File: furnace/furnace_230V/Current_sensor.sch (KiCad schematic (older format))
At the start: 14 parts, among them T1 ZMCT103C

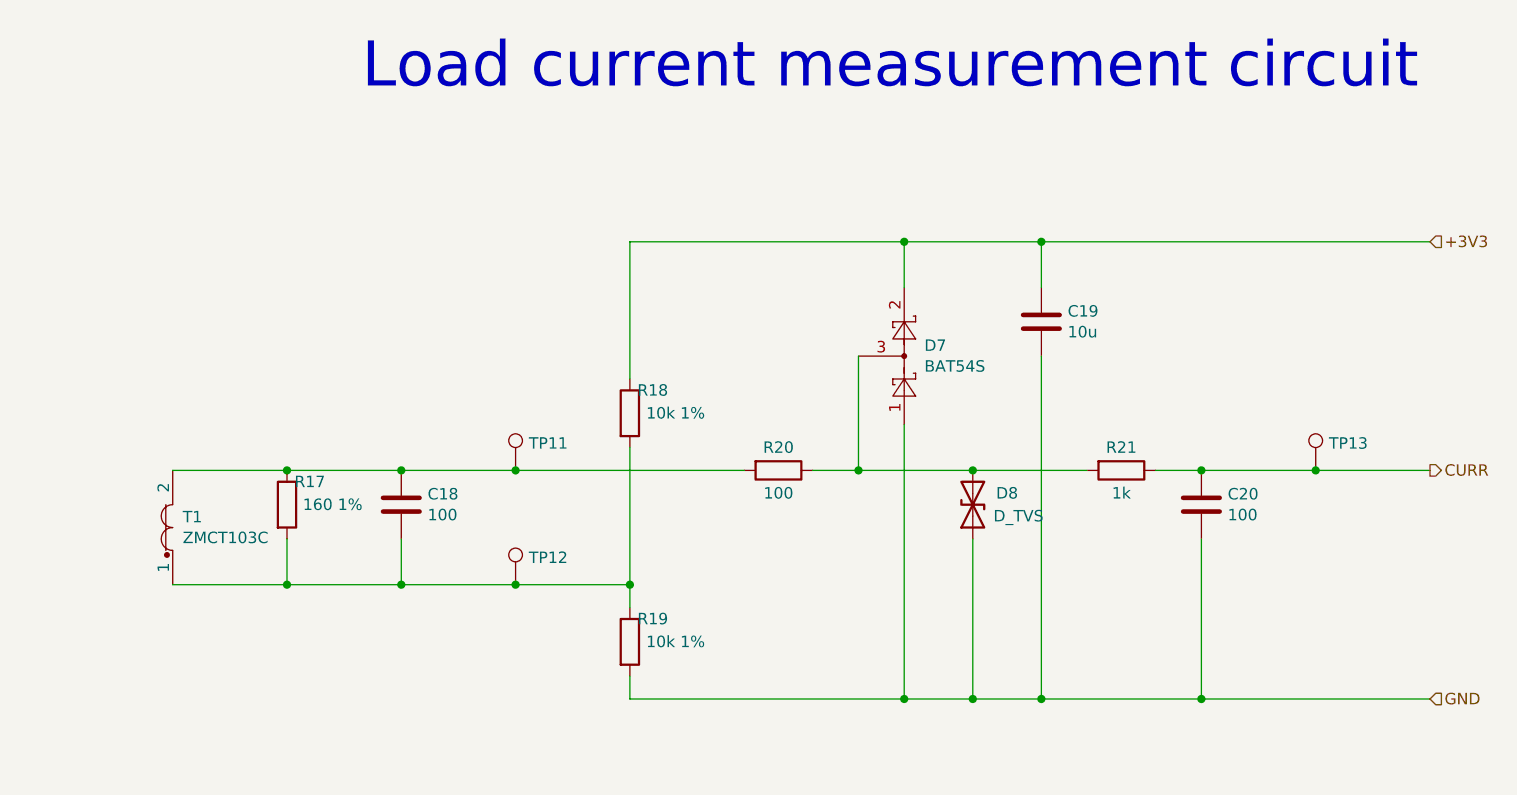
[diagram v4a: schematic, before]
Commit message: Add files via upload
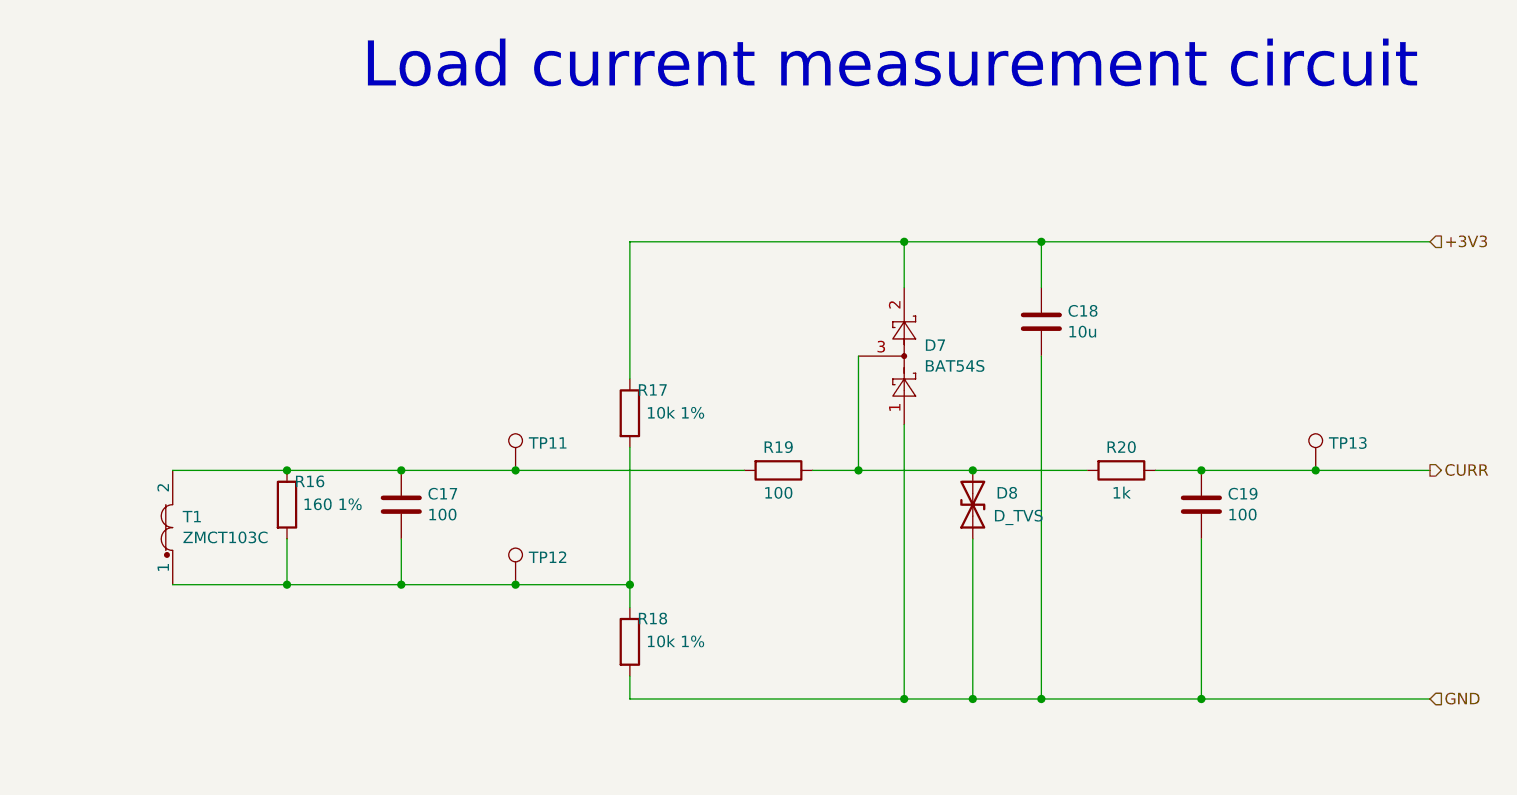
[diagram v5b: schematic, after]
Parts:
- C17: renamed from C18; footprint Capacitor_SMD:C_0603_1608Metric_Pad1.08x0.95mm_HandSolder -> Capacitor_SMD:C_0603_1608Metric_Pad1.05x0.95mm_HandSolder
- C18: renamed from C19; footprint Capacitor_SMD:C_0603_1608Metric_Pad1.08x0.95mm_HandSolder -> Capacitor_SMD:C_0603_1608Metric_Pad1.05x0.95mm_HandSolder
- C19: renamed from C20; footprint Capacitor_SMD:C_0603_1608Metric_Pad1.08x0.95mm_HandSolder -> Capacitor_SMD:C_0603_1608Metric_Pad1.05x0.95mm_HandSolder
- D8: footprint Diode_SMD:D_SMA-SMB_Universal_Handsoldering -> Diode_SMD:D_SMB_Handsoldering
- T1: footprint (none) -> furnace_230V:ZMCT103C
- TP11, TP12, TP13: footprint MountingHole:MountingHole_2.2mm_M2_DIN965_Pad_TopBottom -> furnace_230V:TP
- renumbered R17 to R16, R18 to R17, R19 to R18, R20 to R19, R21 to R20
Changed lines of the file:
@@
 F 0 "TP11" H 4558 4118 50  0000 L CNN
 F 1 "TestPoint" H 4558 4027 50  0001 L CNN
-F 2 "MountingHole:MountingHole_2.2mm_M2_DIN965_Pad_TopBottom" H 4700 4000 50  0001 C CNN
+F 2 "furnace_230V:TP" H 4700 4000 50  0001 C CNN
 F 3 "~" H 4700 4000 50  0001 C CNN
 	1    4500 4000
@@
 F 0 "T1" V 3096 4256 50  0000 R CNN
 F 1 "ZMCT103C" V 3005 4256 50  0000 R CNN
-F 2 "" H 3000 4300 50  0001 C CNN
+F 2 "furnace_230V:ZMCT103C" H 3000 4300 50  0001 C CNN
 F 3 "" H 3000 4300 50  0001 C CNN
 	1    3000 4300
@@
 F 0 "TP12" H 4558 4618 50  0000 L CNN
 F 1 "TestPoint" H 4558 4527 50  0001 L CNN
-F 2 "MountingHole:MountingHole_2.2mm_M2_DIN965_Pad_TopBottom" H 4700 4500 50  0001 C CNN
+F 2 "furnace_230V:TP" H 4700 4500 50  0001 C CNN
 F 3 "~" H 4700 4500 50  0001 C CNN
 	1    4500 4500
@@
 AR Path="/60AAEC6C/60AF1C77" Ref="R?"  Part="1"
 AR Path="/60AAE4BD/60AF1C77" Ref="R?"  Part="1"
-AR Path="/60AAE212/60AF1C77" Ref="R20"  Part="1"
-F 0 "R20" V 5550 4000 50  0000 C CNN
+AR Path="/60AAE212/60AF1C77" Ref="R19"  Part="1"
+F 0 "R19" V 5550 4000 50  0000 C CNN
 F 1 "100" V 5750 4000 50  0000 C CNN
 F 2 "Resistor_SMD:R_0603_1608Metric_Pad1.05x0.95mm_HandSolder" V 5580 4000 50  0001 C CNN
@@
 F 0 "D8" V 6550 4000 50  0000 C CNN
 F 1 "D_TVS" V 6450 3950 50  0000 C CNN
-F 2 "Diode_SMD:D_SMA-SMB_Universal_Handsoldering" H 6500 4150 50  0001 C CNN
+F 2 "Diode_SMD:D_SMB_Handsoldering" H 6500 4150 50  0001 C CNN
 F 3 "~" H 6500 4150 50  0001 C CNN
 	1    6500 4150
@@
 AR Path="/60AAEC6C/60AF1C89" Ref="R?"  Part="1"
 AR Path="/60AAE4BD/60AF1C89" Ref="R?"  Part="1"
-AR Path="/60AAE212/60AF1C89" Ref="R21"  Part="1"
-F 0 "R21" V 7050 4000 50  0000 C CNN
+AR Path="/60AAE212/60AF1C89" Ref="R20"  Part="1"
+F 0 "R20" V 7050 4000 50  0000 C CNN
 F 1 "1k" V 7250 4000 50  0000 C CNN
 F 2 "Resistor_SMD:R_0603_1608Metric_Pad1.05x0.95mm_HandSolder" V 7080 4000 50  0001 C CNN
@@
 AR Path="/60AAC605/60AF1C8F" Ref="C?"  Part="1"
 AR Path="/60AAE4BD/60AF1C8F" Ref="C?"  Part="1"
-AR Path="/60AAE212/60AF1C8F" Ref="C20"  Part="1"
-F 0 "C20" H 7615 4196 50  0000 L CNN
+AR Path="/60AAE212/60AF1C8F" Ref="C19"  Part="1"
+F 0 "C19" H 7615 4196 50  0000 L CNN
 F 1 "100" H 7615 4105 50  0000 L CNN
-F 2 "Capacitor_SMD:C_0603_1608Metric_Pad1.08x0.95mm_HandSolder" H 7538 4000 50  0001 C CNN
+F 2 "Capacitor_SMD:C_0603_1608Metric_Pad1.05x0.95mm_HandSolder" H 7538 4000 50  0001 C CNN
 F 3 "~" H 7500 4150 50  0001 C CNN
 	1    7500 4150
@@
 F 0 "TP13" H 8058 4118 50  0000 L CNN
 F 1 "TestPoint" H 8058 4027 50  0001 L CNN
-F 2 "MountingHole:MountingHole_2.2mm_M2_DIN965_Pad_TopBottom" H 8200 4000 50  0001 C CNN
+F 2 "furnace_230V:TP" H 8200 4000 50  0001 C CNN
 F 3 "~" H 8200 4000 50  0001 C CNN
 	1    8000 4000
@@
 AR Path="/60AAC605/60AF1C9B" Ref="C?"  Part="1"
 AR Path="/60AAE4BD/60AF1C9B" Ref="C?"  Part="1"
-AR Path="/60AAE212/60AF1C9B" Ref="C19"  Part="1"
-F 0 "C19" H 6915 3396 50  0000 L CNN
+AR Path="/60AAE212/60AF1C9B" Ref="C18"  Part="1"
+F 0 "C18" H 6915 3396 50  0000 L CNN
 F 1 "10u" H 6915 3305 50  0000 L CNN
-F 2 "Capacitor_SMD:C_0603_1608Metric_Pad1.08x0.95mm_HandSolder" H 6838 3200 50  0001 C CNN
+F 2 "Capacitor_SMD:C_0603_1608Metric_Pad1.05x0.95mm_HandSolder" H 6838 3200 50  0001 C CNN
 F 3 "~" H 6800 3350 50  0001 C CNN
 	1    6800 3350
@@
 AR Path="/60AAC605/60AF29E2" Ref="C?"  Part="1"
 AR Path="/60AAE4BD/60AF29E2" Ref="C?"  Part="1"
-AR Path="/60AAE212/60AF29E2" Ref="C18"  Part="1"
-F 0 "C18" H 4115 4196 50  0000 L CNN
+AR Path="/60AAE212/60AF29E2" Ref="C17"  Part="1"
+F 0 "C17" H 4115 4196 50  0000 L CNN
 F 1 "100" H 4115 4105 50  0000 L CNN
-F 2 "Capacitor_SMD:C_0603_1608Metric_Pad1.08x0.95mm_HandSolder" H 4038 4000 50  0001 C CNN
+F 2 "Capacitor_SMD:C_0603_1608Metric_Pad1.05x0.95mm_HandSolder" H 4038 4000 50  0001 C CNN
 F 3 "~" H 4000 4150 50  0001 C CNN
 	1    4000 4150
@@
 AR Path="/60AAE0B8/60AF645E" Ref="R?"  Part="1"
 AR Path="/60AAEC6C/60AF645E" Ref="R?"  Part="1"
-AR Path="/60AAE212/60AF645E" Ref="R17"  Part="1"
-F 0 "R17" H 3600 4250 50  0000 C CNN
+AR Path="/60AAE212/60AF645E" Ref="R16"  Part="1"
+F 0 "R16" H 3600 4250 50  0000 C CNN
 F 1 "160 1%" H 3700 4150 50  0000 C CNN
 F 2 "Resistor_SMD:R_0603_1608Metric_Pad1.05x0.95mm_HandSolder" V 3430 4150 50  0001 C CNN
@@
 AR Path="/60AAE0B8/60AFBCF4" Ref="R?"  Part="1"
 AR Path="/60AAEC6C/60AFBCF4" Ref="R?"  Part="1"
-AR Path="/60AAE212/60AFBCF4" Ref="R18"  Part="1"
-F 0 "R18" H 5100 3850 50  0000 C CNN
+AR Path="/60AAE212/60AFBCF4" Ref="R17"  Part="1"
+F 0 "R17" H 5100 3850 50  0000 C CNN
 F 1 "10k 1%" H 5200 3750 50  0000 C CNN
 F 2 "Resistor_SMD:R_0603_1608Metric_Pad1.05x0.95mm_HandSolder" V 4930 3750 50  0001 C CNN
@@
 AR Path="/60AAE0B8/60AFC31E" Ref="R?"  Part="1"
 AR Path="/60AAEC6C/60AFC31E" Ref="R?"  Part="1"
-AR Path="/60AAE212/60AFC31E" Ref="R19"  Part="1"
-F 0 "R19" H 5100 4850 50  0000 C CNN
+AR Path="/60AAE212/60AFC31E" Ref="R18"  Part="1"
+F 0 "R18" H 5100 4850 50  0000 C CNN
 F 1 "10k 1%" H 5200 4750 50  0000 C CNN
 F 2 "Resistor_SMD:R_0603_1608Metric_Pad1.05x0.95mm_HandSolder" V 4930 4750 50  0001 C CNN

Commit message: Add files via upload
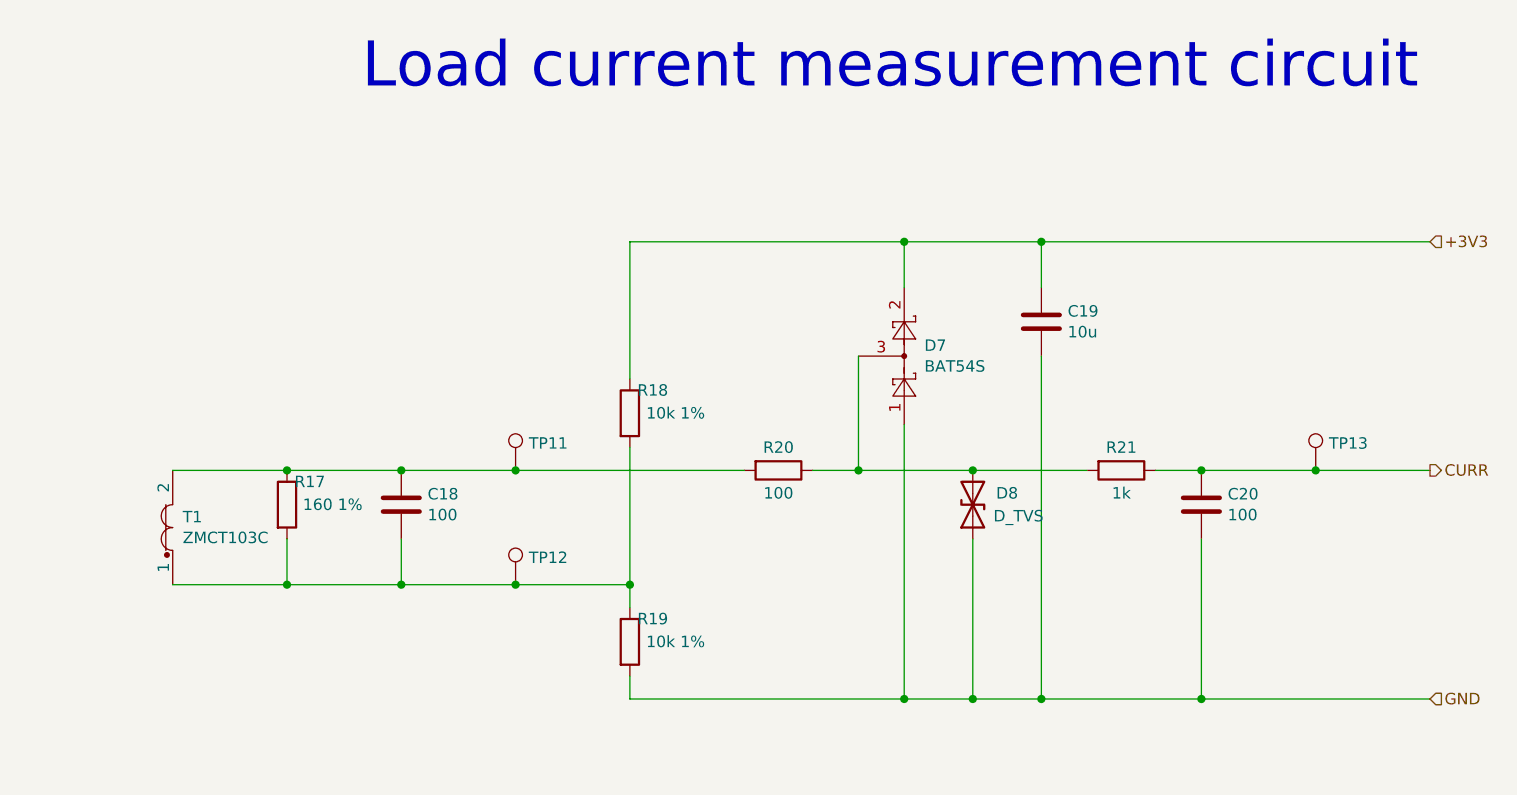
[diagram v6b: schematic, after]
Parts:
- C18: renamed from C17; footprint Capacitor_SMD:C_0603_1608Metric_Pad1.05x0.95mm_HandSolder -> Capacitor_SMD:C_0603_1608Metric_Pad1.08x0.95mm_HandSolder
- C19: renamed from C18; footprint Capacitor_SMD:C_0603_1608Metric_Pad1.05x0.95mm_HandSolder -> Capacitor_SMD:C_0603_1608Metric_Pad1.08x0.95mm_HandSolder
- C20: renamed from C19; footprint Capacitor_SMD:C_0603_1608Metric_Pad1.05x0.95mm_HandSolder -> Capacitor_SMD:C_0603_1608Metric_Pad1.08x0.95mm_HandSolder
- D8: footprint Diode_SMD:D_SMB_Handsoldering -> Diode_SMD:D_SMA-SMB_Universal_Handsoldering
- T1: footprint furnace_230V:ZMCT103C -> (none)
- TP11, TP12, TP13: footprint furnace_230V:TP -> MountingHole:MountingHole_2.2mm_M2_DIN965_Pad_TopBottom
- renumbered R16 to R17, R17 to R18, R18 to R19, R19 to R20, R20 to R21
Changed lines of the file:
@@
 F 0 "TP11" H 4558 4118 50  0000 L CNN
 F 1 "TestPoint" H 4558 4027 50  0001 L CNN
-F 2 "furnace_230V:TP" H 4700 4000 50  0001 C CNN
+F 2 "MountingHole:MountingHole_2.2mm_M2_DIN965_Pad_TopBottom" H 4700 4000 50  0001 C CNN
 F 3 "~" H 4700 4000 50  0001 C CNN
 	1    4500 4000
@@
 F 0 "T1" V 3096 4256 50  0000 R CNN
 F 1 "ZMCT103C" V 3005 4256 50  0000 R CNN
-F 2 "furnace_230V:ZMCT103C" H 3000 4300 50  0001 C CNN
+F 2 "" H 3000 4300 50  0001 C CNN
 F 3 "" H 3000 4300 50  0001 C CNN
 	1    3000 4300
@@
 F 0 "TP12" H 4558 4618 50  0000 L CNN
 F 1 "TestPoint" H 4558 4527 50  0001 L CNN
-F 2 "furnace_230V:TP" H 4700 4500 50  0001 C CNN
+F 2 "MountingHole:MountingHole_2.2mm_M2_DIN965_Pad_TopBottom" H 4700 4500 50  0001 C CNN
 F 3 "~" H 4700 4500 50  0001 C CNN
 	1    4500 4500
@@
 AR Path="/60AAEC6C/60AF1C77" Ref="R?"  Part="1"
 AR Path="/60AAE4BD/60AF1C77" Ref="R?"  Part="1"
-AR Path="/60AAE212/60AF1C77" Ref="R19"  Part="1"
-F 0 "R19" V 5550 4000 50  0000 C CNN
+AR Path="/60AAE212/60AF1C77" Ref="R20"  Part="1"
+F 0 "R20" V 5550 4000 50  0000 C CNN
 F 1 "100" V 5750 4000 50  0000 C CNN
 F 2 "Resistor_SMD:R_0603_1608Metric_Pad1.05x0.95mm_HandSolder" V 5580 4000 50  0001 C CNN
@@
 F 0 "D8" V 6550 4000 50  0000 C CNN
 F 1 "D_TVS" V 6450 3950 50  0000 C CNN
-F 2 "Diode_SMD:D_SMB_Handsoldering" H 6500 4150 50  0001 C CNN
+F 2 "Diode_SMD:D_SMA-SMB_Universal_Handsoldering" H 6500 4150 50  0001 C CNN
 F 3 "~" H 6500 4150 50  0001 C CNN
 	1    6500 4150
@@
 AR Path="/60AAEC6C/60AF1C89" Ref="R?"  Part="1"
 AR Path="/60AAE4BD/60AF1C89" Ref="R?"  Part="1"
-AR Path="/60AAE212/60AF1C89" Ref="R20"  Part="1"
-F 0 "R20" V 7050 4000 50  0000 C CNN
+AR Path="/60AAE212/60AF1C89" Ref="R21"  Part="1"
+F 0 "R21" V 7050 4000 50  0000 C CNN
 F 1 "1k" V 7250 4000 50  0000 C CNN
 F 2 "Resistor_SMD:R_0603_1608Metric_Pad1.05x0.95mm_HandSolder" V 7080 4000 50  0001 C CNN
@@
 AR Path="/60AAC605/60AF1C8F" Ref="C?"  Part="1"
 AR Path="/60AAE4BD/60AF1C8F" Ref="C?"  Part="1"
-AR Path="/60AAE212/60AF1C8F" Ref="C19"  Part="1"
-F 0 "C19" H 7615 4196 50  0000 L CNN
+AR Path="/60AAE212/60AF1C8F" Ref="C20"  Part="1"
+F 0 "C20" H 7615 4196 50  0000 L CNN
 F 1 "100" H 7615 4105 50  0000 L CNN
-F 2 "Capacitor_SMD:C_0603_1608Metric_Pad1.05x0.95mm_HandSolder" H 7538 4000 50  0001 C CNN
+F 2 "Capacitor_SMD:C_0603_1608Metric_Pad1.08x0.95mm_HandSolder" H 7538 4000 50  0001 C CNN
 F 3 "~" H 7500 4150 50  0001 C CNN
 	1    7500 4150
@@
 F 0 "TP13" H 8058 4118 50  0000 L CNN
 F 1 "TestPoint" H 8058 4027 50  0001 L CNN
-F 2 "furnace_230V:TP" H 8200 4000 50  0001 C CNN
+F 2 "MountingHole:MountingHole_2.2mm_M2_DIN965_Pad_TopBottom" H 8200 4000 50  0001 C CNN
 F 3 "~" H 8200 4000 50  0001 C CNN
 	1    8000 4000
@@
 AR Path="/60AAC605/60AF1C9B" Ref="C?"  Part="1"
 AR Path="/60AAE4BD/60AF1C9B" Ref="C?"  Part="1"
-AR Path="/60AAE212/60AF1C9B" Ref="C18"  Part="1"
-F 0 "C18" H 6915 3396 50  0000 L CNN
+AR Path="/60AAE212/60AF1C9B" Ref="C19"  Part="1"
+F 0 "C19" H 6915 3396 50  0000 L CNN
 F 1 "10u" H 6915 3305 50  0000 L CNN
-F 2 "Capacitor_SMD:C_0603_1608Metric_Pad1.05x0.95mm_HandSolder" H 6838 3200 50  0001 C CNN
+F 2 "Capacitor_SMD:C_0603_1608Metric_Pad1.08x0.95mm_HandSolder" H 6838 3200 50  0001 C CNN
 F 3 "~" H 6800 3350 50  0001 C CNN
 	1    6800 3350
@@
 AR Path="/60AAC605/60AF29E2" Ref="C?"  Part="1"
 AR Path="/60AAE4BD/60AF29E2" Ref="C?"  Part="1"
-AR Path="/60AAE212/60AF29E2" Ref="C17"  Part="1"
-F 0 "C17" H 4115 4196 50  0000 L CNN
+AR Path="/60AAE212/60AF29E2" Ref="C18"  Part="1"
+F 0 "C18" H 4115 4196 50  0000 L CNN
 F 1 "100" H 4115 4105 50  0000 L CNN
-F 2 "Capacitor_SMD:C_0603_1608Metric_Pad1.05x0.95mm_HandSolder" H 4038 4000 50  0001 C CNN
+F 2 "Capacitor_SMD:C_0603_1608Metric_Pad1.08x0.95mm_HandSolder" H 4038 4000 50  0001 C CNN
 F 3 "~" H 4000 4150 50  0001 C CNN
 	1    4000 4150
@@
 AR Path="/60AAE0B8/60AF645E" Ref="R?"  Part="1"
 AR Path="/60AAEC6C/60AF645E" Ref="R?"  Part="1"
-AR Path="/60AAE212/60AF645E" Ref="R16"  Part="1"
-F 0 "R16" H 3600 4250 50  0000 C CNN
+AR Path="/60AAE212/60AF645E" Ref="R17"  Part="1"
+F 0 "R17" H 3600 4250 50  0000 C CNN
 F 1 "160 1%" H 3700 4150 50  0000 C CNN
 F 2 "Resistor_SMD:R_0603_1608Metric_Pad1.05x0.95mm_HandSolder" V 3430 4150 50  0001 C CNN
@@
 AR Path="/60AAE0B8/60AFBCF4" Ref="R?"  Part="1"
 AR Path="/60AAEC6C/60AFBCF4" Ref="R?"  Part="1"
-AR Path="/60AAE212/60AFBCF4" Ref="R17"  Part="1"
-F 0 "R17" H 5100 3850 50  0000 C CNN
+AR Path="/60AAE212/60AFBCF4" Ref="R18"  Part="1"
+F 0 "R18" H 5100 3850 50  0000 C CNN
 F 1 "10k 1%" H 5200 3750 50  0000 C CNN
 F 2 "Resistor_SMD:R_0603_1608Metric_Pad1.05x0.95mm_HandSolder" V 4930 3750 50  0001 C CNN
@@
 AR Path="/60AAE0B8/60AFC31E" Ref="R?"  Part="1"
 AR Path="/60AAEC6C/60AFC31E" Ref="R?"  Part="1"
-AR Path="/60AAE212/60AFC31E" Ref="R18"  Part="1"
-F 0 "R18" H 5100 4850 50  0000 C CNN
+AR Path="/60AAE212/60AFC31E" Ref="R19"  Part="1"
+F 0 "R19" H 5100 4850 50  0000 C CNN
 F 1 "10k 1%" H 5200 4750 50  0000 C CNN
 F 2 "Resistor_SMD:R_0603_1608Metric_Pad1.05x0.95mm_HandSolder" V 4930 4750 50  0001 C CNN
